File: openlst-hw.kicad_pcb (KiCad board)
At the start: 4 copper layers, 60 x 50 mm, 175 parts, among them J1 5VDC, J2 CC Prog/Debug, J3 UART0, J4 UART1, J5 Control Outputs, J6 ANT, U1 LM1117-3.3, U2 CC1110, U3 LT1086-3.6, U4 FOX924 27MHz, U5 TLV803S, U6 PE4259, U8 STA1120A, U9 RFFM6403

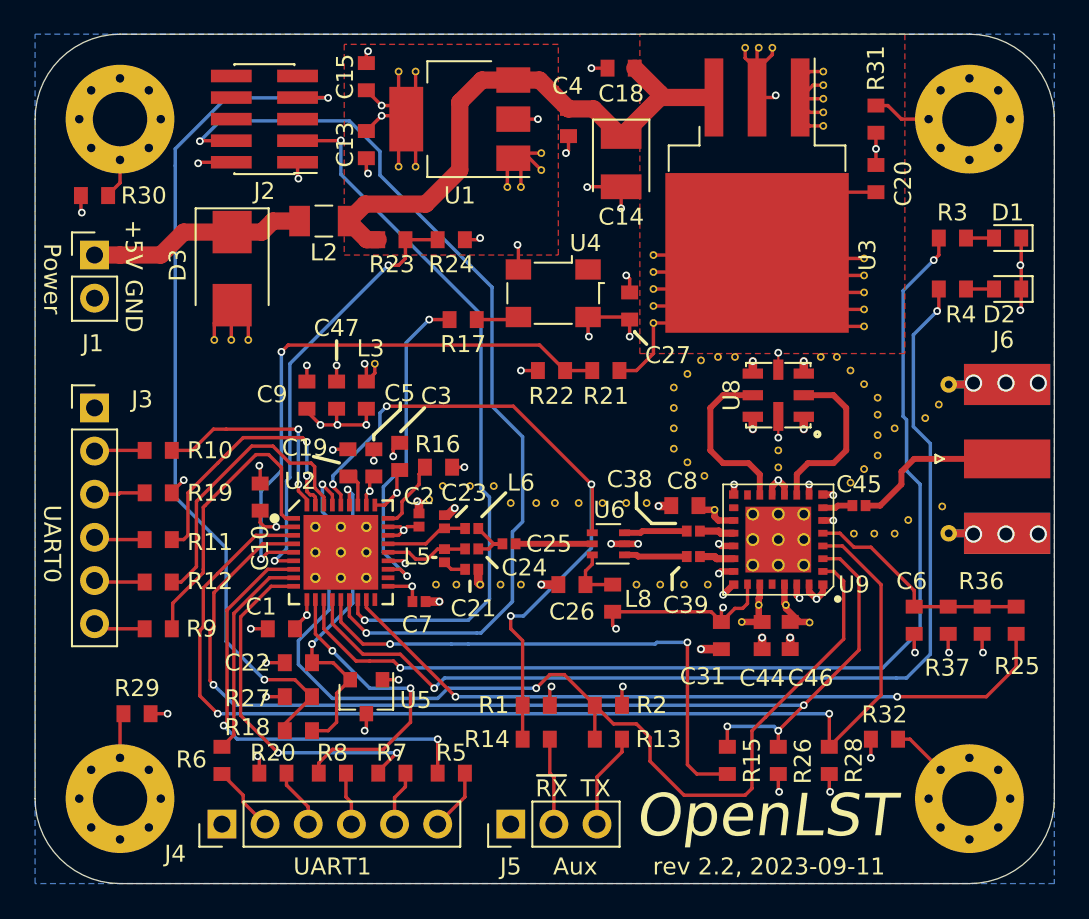
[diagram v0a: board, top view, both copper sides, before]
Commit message: DRC cleanup
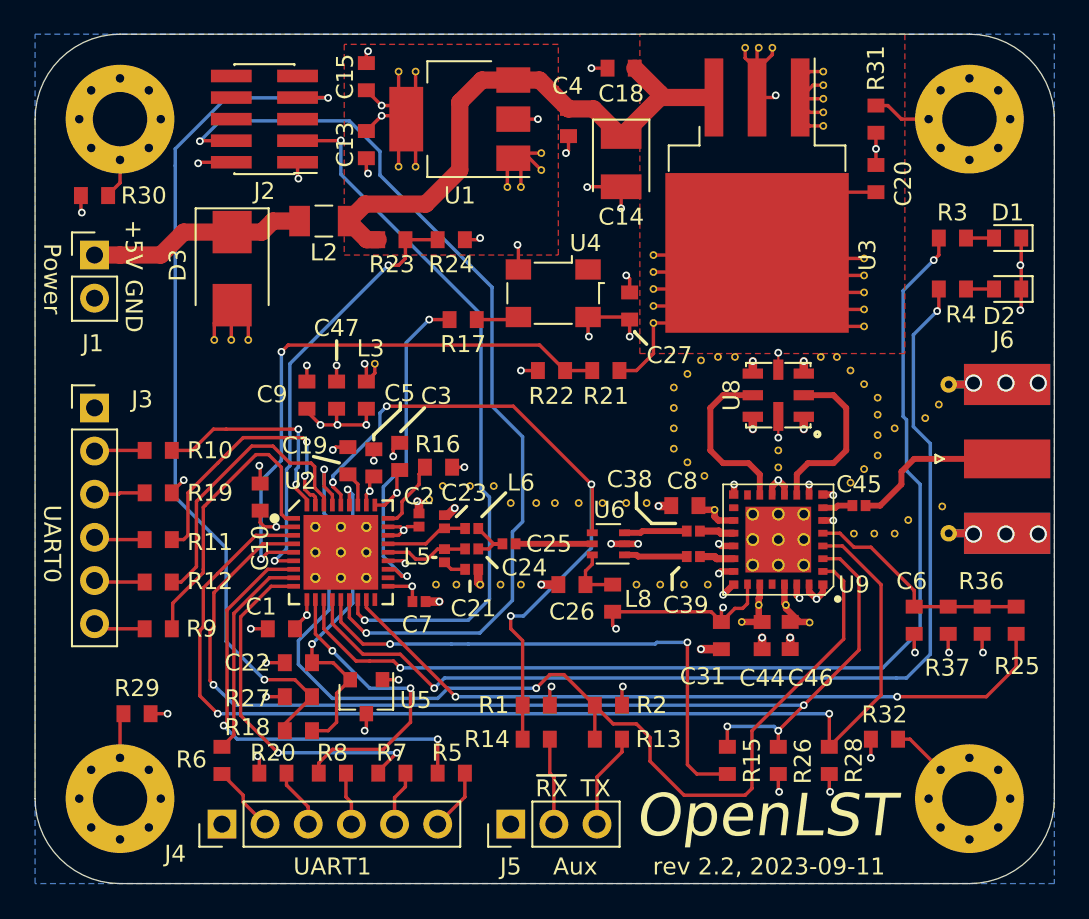
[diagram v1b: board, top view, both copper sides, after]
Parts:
- moved C19 0.13 mm to (131.9, 63.6)
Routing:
- net /LST_TX_MODE: track 63.3 -> 64.5 mm
